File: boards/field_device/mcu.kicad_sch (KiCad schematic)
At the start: 19 parts, among them J1 Conn_01x05_Pin, J2 Conn_01x02_Pin, SW1 SW_SPST, U2 STM32C051F6P6

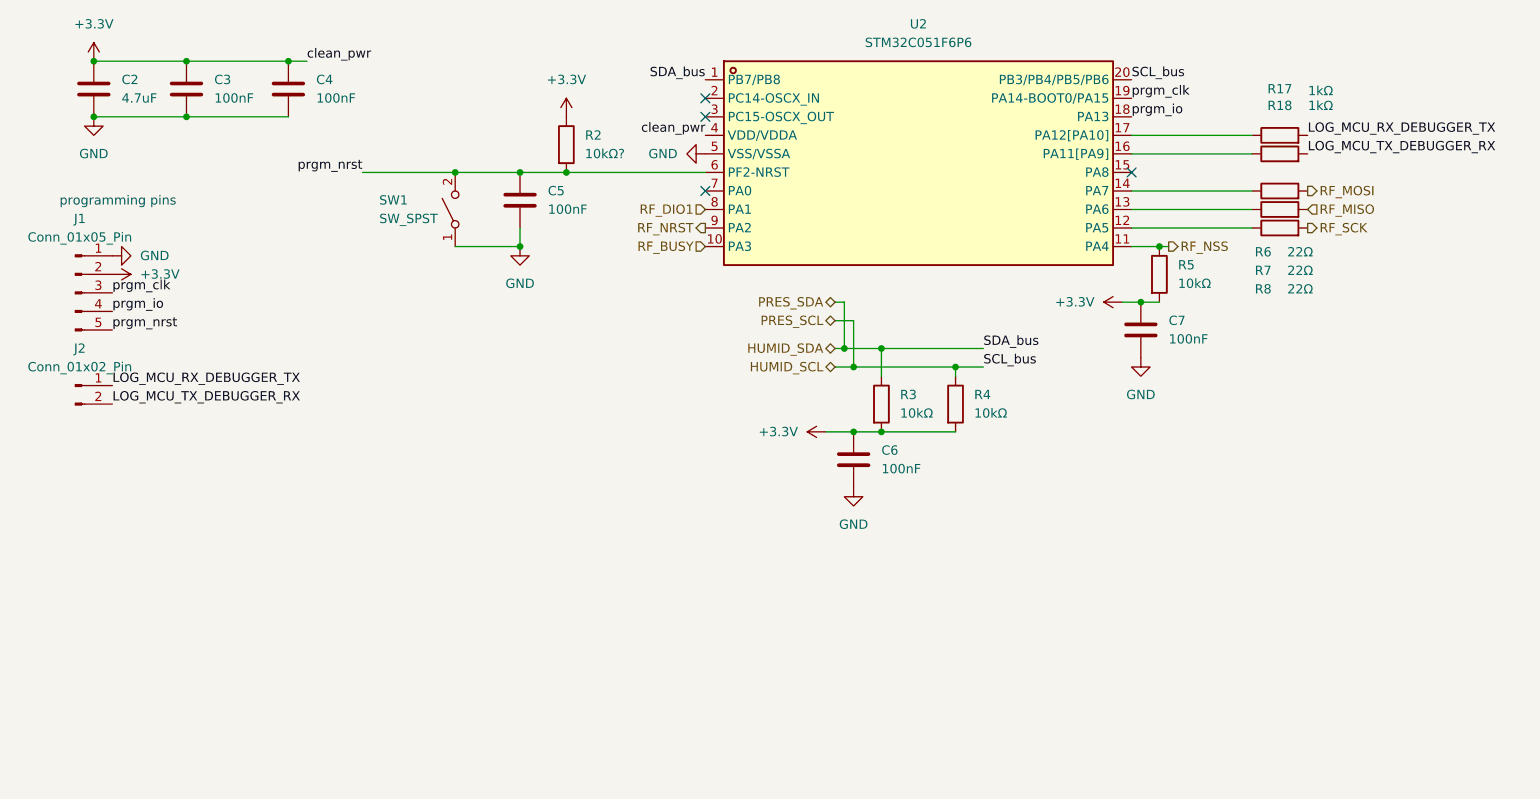
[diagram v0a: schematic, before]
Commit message: reorganized mcu
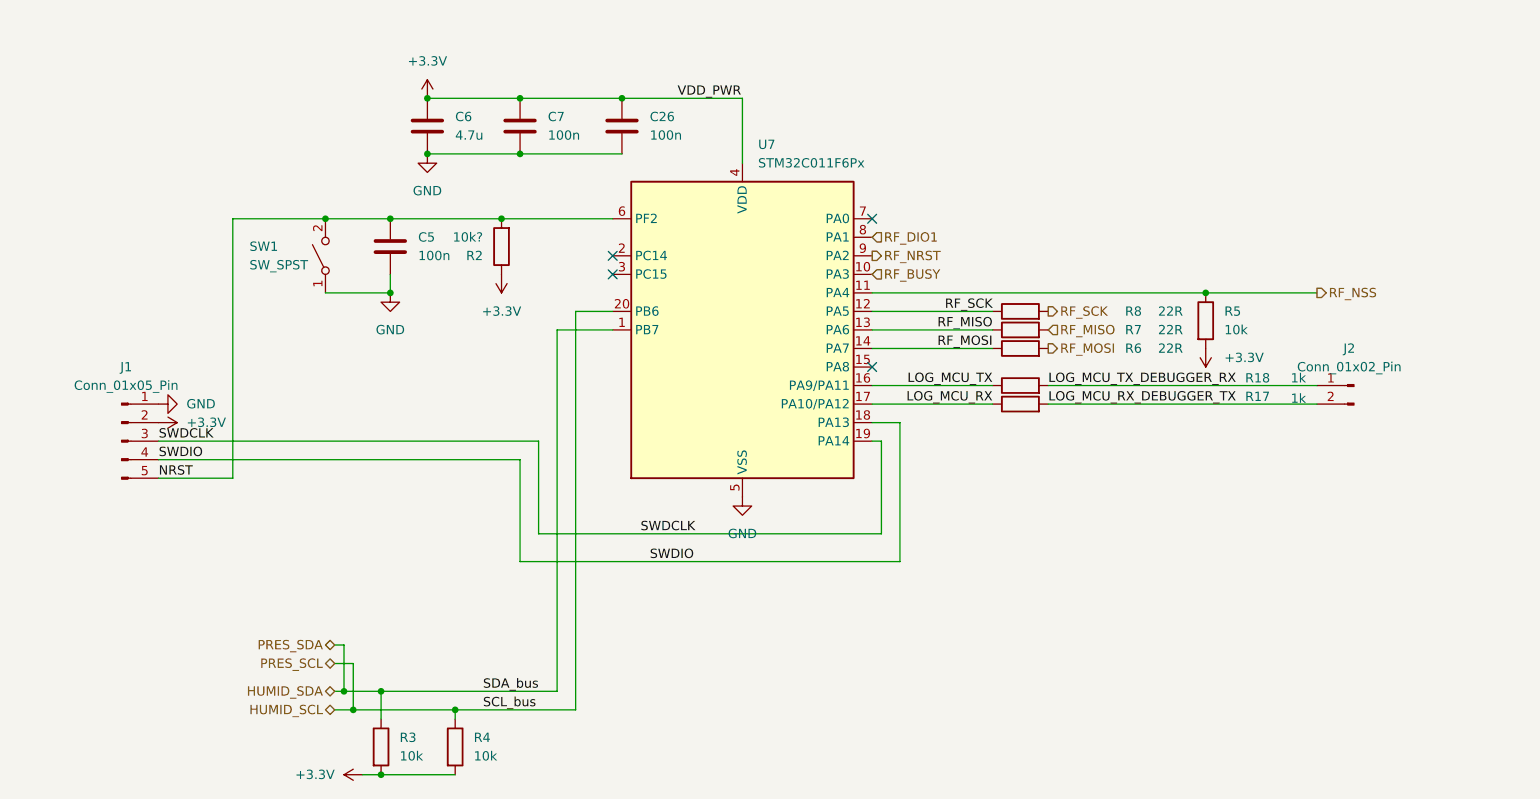
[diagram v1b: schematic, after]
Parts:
- removed C2: 4.7uF, Capacitor_SMD:C_0603_1608Metric, symbol Device:C
- removed C3, C4: 100nF, Capacitor_SMD:C_0603_1608Metric, symbol Device:C
- removed U2: STM32C051F6P6, LCSC downloads:TSSOP-20_L6.5-W4.4-P0.65-LS6.4-BL, symbol lcsc downloads:STM32C051F6P6
- added C26: 100n, Capacitor_SMD:C_0603_1608Metric, symbol Device:C
- added U7: STM32C011F6Px, Package_SO:TSSOP-20_4.4x6.5mm_P0.65mm, symbol MCU_ST_STM32C0:STM32C011F6Px
- C5, C7: value 100nF -> 100n
- C6: value 100nF -> 4.7u
- R17, R18: value 1kΩ -> 1k
- R2: value 10kΩ? -> 10k?
- R3, R4, R5: value 10kΩ -> 10k
- R6, R7, R8: value 22Ω -> 22R
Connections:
- net +3.3V: now also C26.1, U7.4 (VDD)
- net GND: now also C26.2, U7.5 (VSS)
- net HUMID_SCL: now also U7.20 (PB6)
- net HUMID_SDA: now also U7.1 (PB7)
- net LOG_MCU_RX_DEBUGGER_TX: now also J2.2 (Pin_2); no longer J2.1 (Pin_1)
- net LOG_MCU_TX_DEBUGGER_RX: now also J2.1 (Pin_1); no longer J2.2 (Pin_2)
- net RF_BUSY: now also U7.10 (PA3)
- net RF_DIO1: now also U7.8 (PA1)
- net RF_MISO: now also R7.1, U7.13 (PA6)
- net RF_MOSI: now also R6.1, U7.14 (PA7)
- net RF_NRST: now also U7.9 (PA2)
- net RF_NSS: now also U7.11 (PA4)
- net RF_SCK: now also R8.1, U7.12 (PA5)
- net LOG_MCU_TX: now reaches R18.1
- net LOG_MCU_TX: now also U7.16 (PA9/PA11)
- net LOG_MCU_RX: now reaches R17.1
- net LOG_MCU_RX: now also U7.17 (PA10/PA12)
- net prgm_clk renamed SWDCLK
- net SWDCLK: now also U7.19 (PA14)
- net prgm_io renamed SWDIO
- net SWDIO: now also U7.18 (PA13)
- net prgm_nrst renamed NRST
- net NRST: now also U7.6 (PF2)
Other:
- note removed: "programming pins"
- moved on the sheet: C5, J1, J2, R17, R18, R2, R3, R4, R5, R6, R7, R8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
